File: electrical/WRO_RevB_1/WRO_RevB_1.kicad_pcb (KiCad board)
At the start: 2 copper layers, 117.5 x 50.6 mm, 23 parts, among them J1 VCC, J2 Conn_01x04_Pin, J4 Conn_01x11_Pin, J5 Conn_01x11_Pin, J6 3v3, J8 Conn_01x04_Pin, SW1 EXEC_PRGM, SW2 PWR, U3 BOB-12009

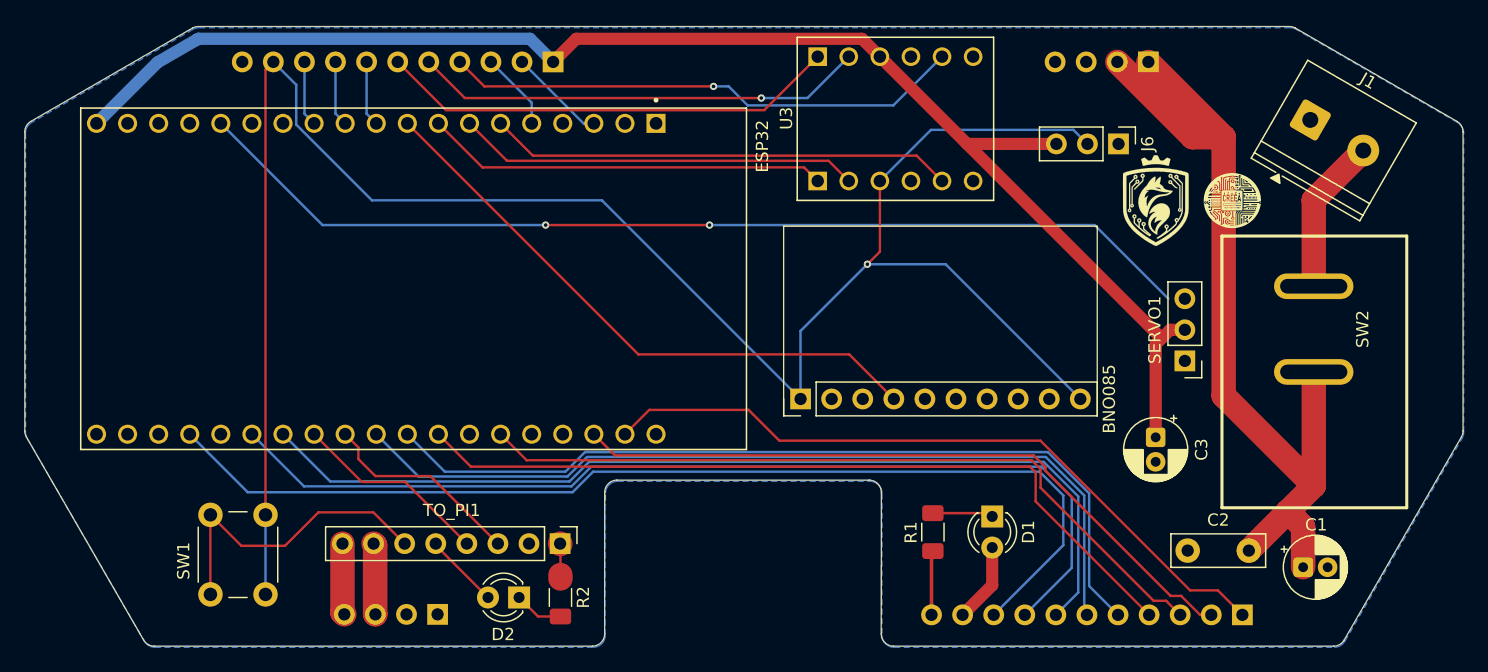
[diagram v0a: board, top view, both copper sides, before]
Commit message: actualiza PCB RevB
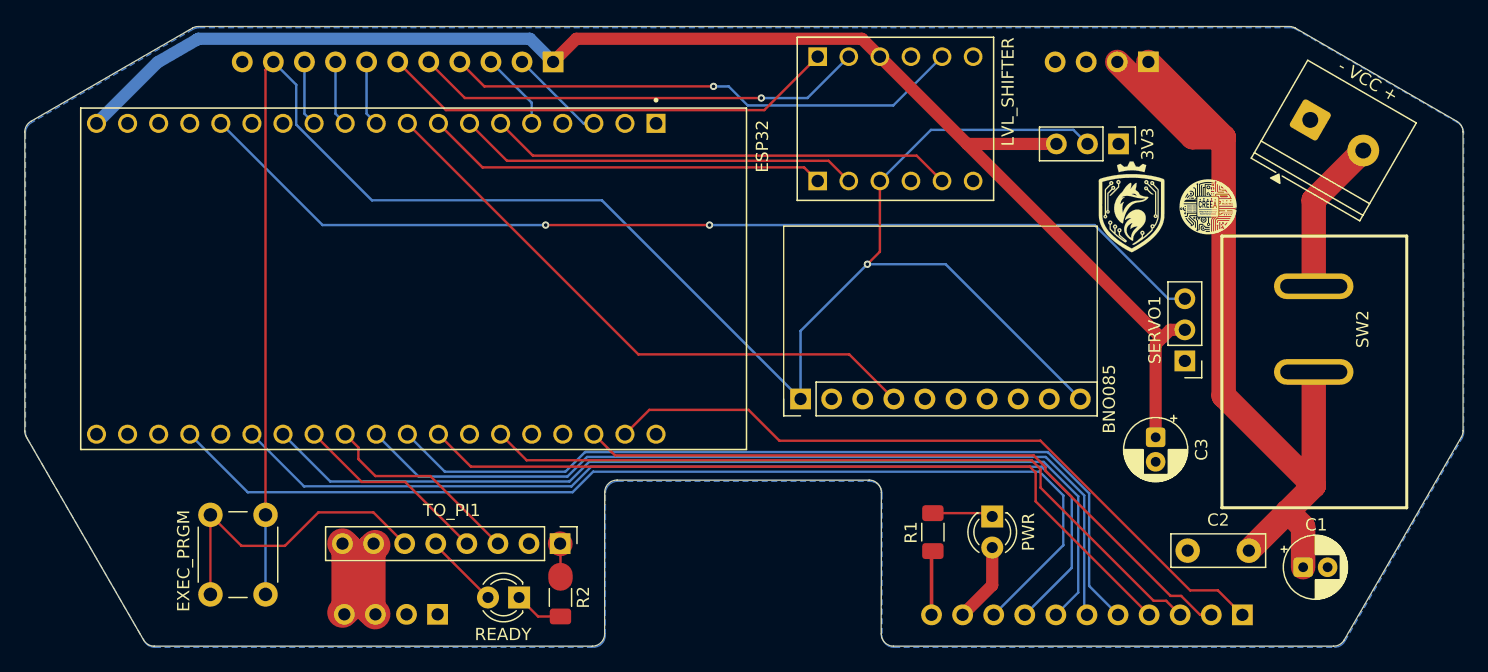
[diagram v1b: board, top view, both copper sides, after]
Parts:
- - VCC +: renamed from J1
- moved G*** 2.04 mm to (182.0, 81.5)
- moved G*** 2.04 mm to (188.2, 81.3)
- renumbered J6 to 3V3, SW1 to EXEC_PRGM, U3 to LVL_SHIFTER, D1 to PWR, D2 to READY
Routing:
- net SERVO: track 83.4 -> 84.7 mm
- net +5V_PI: track 11.7 -> 12.3 mm
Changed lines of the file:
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@@
 		(descr "Terminal Block Phoenix PT-1,5-2-5.0-H, 2 pins, pitch 5mm, size 10x9mm, drill diameter 1.3mm, pad diameter 2.6mm, http://www.mouser.com/ds/2/324/ItemDetail_1935161-922578.pdf")
 		(tags "THT Terminal Block Phoenix PT-1,5-2-5.0-H pitch 5mm size 10x9mm drill 1.3mm pad 2.6mm")
-		(property "Reference" "J1"
+		(property "Reference" "- VCC +"
 			(at 2.500001 -5.119999 150)
 			(layer "F.SilkS")
@@
 		(descr "Through hole straight pin header, 1x03, 2.54mm pitch, single row")
 		(tags "Through hole pin header THT 1x03 2.54mm single row")
-		(property "Reference" "J6"
+		(property "Reference" "3V3"
 			(at 0 -2.38 90)
 			(layer "F.SilkS")
@@
 		(layer "F.Cu")
 		(at 162.67 74.13 90)
-		(property "Reference" "U3"
-			(at 0.04 -8.9125 90)
+		(property "Reference" "LVL_SHIFTER"
+			(at 2.21 9.2 90)
 			(layer "F.SilkS")
 			(effects
@@
 	(footprint "LogoCREEA:LogoCREEA4.5"
 		(layer "F.Cu")
-		(at 190.22 80.812297)
+		(at 188.242289 81.319751)
 		(property "Reference" "G***"
 			(at 0 0 0)
@@
 		(descr "LED, diameter 3.0mm, 2 pins, generated by kicad-footprint-generator")
 		(tags "LED")
-		(property "Reference" "D2"
+		(property "Reference" "READY"
 			(at 1.31 -3.02 0)
 			(layer "F.SilkS")
@@
 		(descr "Generic 6mm SW tactile push button")
 		(tags "tact sw push 6mm")
-		(property "Reference" "SW1"
+		(property "Reference" "EXEC_PRGM"
 			(at 3.76 6.69 90)
 			(layer "F.SilkS")
@@
 	(footprint "LogoFoxR_2:LogoFoxR_2"
 		(layer "F.Cu")
-		(at 183.948975 80.959751)
+		(at 181.971264 81.467205)
 		(property "Reference" "G***"
 			(at 0 0 0)
@@
 		(descr "LED, diameter 3.0mm, 2 pins, generated by kicad-footprint-generator")
 		(tags "LED")
-		(property "Reference" "D1"
+		(property "Reference" "PWR"
 			(at 1.27 -2.96 90)
 			(layer "F.SilkS")
@@
 	)
 	(segment
-		(start 120.16 108.97)
-		(end 120.16 114.6)
-		(width 2)
+		(start 117.49 108.84)
+		(end 117.83 109.18)
+		(width 2.5)
+		(layer "F.Cu")
+		(net "+5V_PI")
+	)
+	(segment
+		(start 117.83 109.18)
+		(end 117.83 114.13)
+		(width 2.5)
+		(layer "F.Cu")
+		(net "+5V_PI")
+	)
+	(segment
+		(start 119.76 109.37)
+		(end 119.76 114.2)
+		(width 2.5)
 		(layer "F.Cu")
 		(net "+5V_PI")
@@
 	)
 	(segment
+		(start 117.83 114.13)
+		(end 117.49 114.47)
+		(width 2.5)
+		(layer "F.Cu")
+		(net "+5V_PI")
+	)
+	(segment
+		(start 120.16 108.97)
+		(end 119.76 109.37)
+		(width 2.5)
+		(layer "F.Cu")
+		(net "+5V_PI")
+	)
+	(segment
 		(start 117.49 114.47)
 		(end 117.64 114.62)
@@
 	)
 	(segment
-		(start 117.49 108.84)
-		(end 117.49 114.47)
-		(width 2)
+		(start 119.76 114.2)
+		(end 120.16 114.6)
+		(width 2.5)
 		(layer "F.Cu")
 		(net "+5V_PI")
 	)
 	(segment
+		(start 170.58 112.24)
+		(end 168.16 114.66)
+		(width 1)
+		(layer "F.Cu")
+		(net "+5V")
+	)
+	(segment
+		(start 184.35396 92.00396)
+		(end 168.53 76.18)
+		(width 1)
+		(layer "F.Cu")
+		(net "+5V")
+	)
+	(segment
+		(start 185.117919 91.37)
+		(end 186.32 91.37)
+		(width 1)
+		(layer "F.Cu")
+		(net "+5V")
+	)
+	(segment
+		(start 175.82 76.18)
+		(end 168.53 76.18)
+		(width 1)
+		(layer "F.Cu")
+		(net "+5V")
+	)
+	(segment
+		(start 184.48396 92.00396)
+		(end 184.35396 92.00396)
+		(width 1)
+		(layer "F.Cu")
+		(net "+5V")
+	)
+	(segment
+		(start 161.4 69.05)
+		(end 168.53 76.18)
+		(width 1)
+		(layer "F.Cu")
+		(net "+5V")
+	)
+	(segment
+		(start 170.58 109.16)
+		(end 170.58 112.24)
+		(width 1)
+		(layer "F.Cu")
+		(net "+5V")
+	)
+	(segment
+		(start 183.935 92.552919)
+		(end 184.48396 92.00396)
+		(width 1)
+		(layer "F.Cu")
+		(net "+5V")
+	)
+	(segment
+		(start 134.7 69.48)
+		(end 136.592 67.588)
+		(width 1)
+		(layer "F.Cu")
+		(net "+5V")
+	)
+	(segment
+		(start 183.935 100.154775)
+		(end 183.935 92.552919)
+		(width 1)
+		(layer "F.Cu")
+		(net "+5V")
+	)
+	(segment
+		(start 159.938 67.588)
+		(end 161.4 69.05)
+		(width 1)
+		(layer "F.Cu")
+		(net "+5V")
+	)
+	(segment
+		(start 136.592 67.588)
+		(end 159.938 67.588)
+		(width 1)
+		(layer "F.Cu")
+		(net "+5V")
+	)
+	(segment
+		(start 184.48396 92.00396)
+		(end 185.117919 91.37)
+		(width 1)
+		(layer "F.Cu")
+		(net "+5V")
+	)
+	(segment
+		(start 97.39 74.5)
+		(end 102.36696 69.52304)
+		(width 1)
+		(layer "B.Cu")
+		(net "+5V")
+	)
+	(segment
+		(start 105.706797 67.59974)
+		(end 105.719037 67.5875)
+		(width 1)
+		(layer "B.Cu")
+		(net "+5V")
+	)
+	(segment
+		(start 105.719037 67.5875)
+		(end 132.8075 67.5875)
+		(width 1)
+		(layer "B.Cu")
+		(net "+5V")
+	)
+	(segment
+		(start 102.36696 69.52304)
+		(end 105.559653 67.678985)
+		(width 1)
+		(layer "B.Cu")
+		(net "+5V")
+	)
+	(segment
+		(start 132.8075 67.5875)
+		(end 134.7 69.48)
+		(width 1)
+		(layer "B.Cu")
+		(net "+5V")
+	)
+	(segment
+		(start 105.559653 67.678985)
+		(end 105.706797 67.59974)
+		(width 1)
+		(layer "B.Cu")
+		(net "+5V")
+	)
+	(segment
 		(start 200.900127 76.72)
 		(end 196.85 80.770127)
@@
 	)
 	(segment
-		(start 178.95 82.81)
-		(end 147.48 82.81)
-		(width 0.2)
-		(layer "B.Cu")
-		(net "SERVO")
-	)
-	(segment
 		(start 134.09 82.81)
 		(end 115.86 82.81)
@@
 	)
 	(segment
-		(start 184.97 88.83)
-		(end 178.95 82.81)
+		(start 186.32 88.83)
+		(end 184.97 88.83)
 		(width 0.2)
 		(layer "B.Cu")
@@
 	)
 	(segment
-		(start 170.58 112.24)
-		(end 168.16 114.66)
-		(width 1)
-		(layer "F.Cu")
-		(net "+5V")
-	)
-	(segment
-		(start 184.35396 92.00396)
-		(end 168.53 76.18)
-		(width 1)
-		(layer "F.Cu")
-		(net "+5V")
-	)
-	(segment
-		(start 185.117919 91.37)
-		(end 186.32 91.37)
-		(width 1)
-		(layer "F.Cu")
-		(net "+5V")
-	)
-	(segment
-		(start 175.82 76.18)
-		(end 168.53 76.18)
-		(width 1)
-		(layer "F.Cu")
-		(net "+5V")
-	)
-	(segment
-		(start 184.48396 92.00396)
-		(end 184.35396 92.00396)
-		(width 1)
-		(layer "F.Cu")
-		(net "+5V")
-	)
-	(segment
-		(start 161.4 69.05)
-		(end 168.53 76.18)
-		(width 1)
-		(layer "F.Cu")
-		(net "+5V")
-	)
-	(segment
-		(start 170.58 109.16)
-		(end 170.58 112.24)
-		(width 1)
-		(layer "F.Cu")
-		(net "+5V")
-	)
-	(segment
-		(start 183.935 92.552919)
-		(end 184.48396 92.00396)
-		(width 1)
-		(layer "F.Cu")
-		(net "+5V")
-	)
-	(segment
-		(start 134.7 69.48)
-		(end 136.592 67.588)
-		(width 1)
-		(layer "F.Cu")
-		(net "+5V")
-	)
-	(segment
-		(start 183.935 100.154775)
-		(end 183.935 92.552919)
-		(width 1)
-		(layer "F.Cu")
-		(net "+5V")
-	)
-	(segment
-		(start 159.938 67.588)
-		(end 161.4 69.05)
-		(width 1)
-		(layer "F.Cu")
-		(net "+5V")
-	)
-	(segment
-		(start 136.592 67.588)
-		(end 159.938 67.588)
-		(width 1)
-		(layer "F.Cu")
-		(net "+5V")
-	)
-	(segment
-		(start 184.48396 92.00396)
-		(end 185.117919 91.37)
-		(width 1)
-		(layer "F.Cu")
-		(net "+5V")
-	)
-	(segment
-		(start 97.39 74.5)
-		(end 102.36696 69.52304)
-		(width 1)
-		(layer "B.Cu")
-		(net "+5V")
-	)
-	(segment
-		(start 105.706797 67.59974)
-		(end 105.719037 67.5875)
-		(width 1)
-		(layer "B.Cu")
-		(net "+5V")
-	)
-	(segment
-		(start 105.719037 67.5875)
-		(end 132.8075 67.5875)
-		(width 1)
-		(layer "B.Cu")
-		(net "+5V")
-	)
-	(segment
-		(start 102.36696 69.52304)
-		(end 105.559653 67.678985)
-		(width 1)
-		(layer "B.Cu")
-		(net "+5V")
-	)
-	(segment
-		(start 132.8075 67.5875)
-		(end 134.7 69.48)
-		(width 1)
+		(start 184.97 88.83)
+		(end 178.95 82.81)
+		(width 0.2)
 		(layer "B.Cu")
-		(net "+5V")
+		(net "SERVO")
 	)
 	(segment
-		(start 105.559653 67.678985)
-		(end 105.706797 67.59974)
-		(width 1)
+		(start 178.95 82.81)
+		(end 147.48 82.81)
+		(width 0.2)
 		(layer "B.Cu")
-		(net "+5V")
+		(net "SERVO")
 	)
 	(segment

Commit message: Revert "Merge branch 'main' of https://github.com/Nakashima26/WRO_FE_2026_FoxRobotics"
This reverts commit 232f9ecb01216201165b5abf43ae09e229c3eea8, reversing
changes made to 212c0f9856f89e84f48e320d89d4fd8fc24ab9e3.
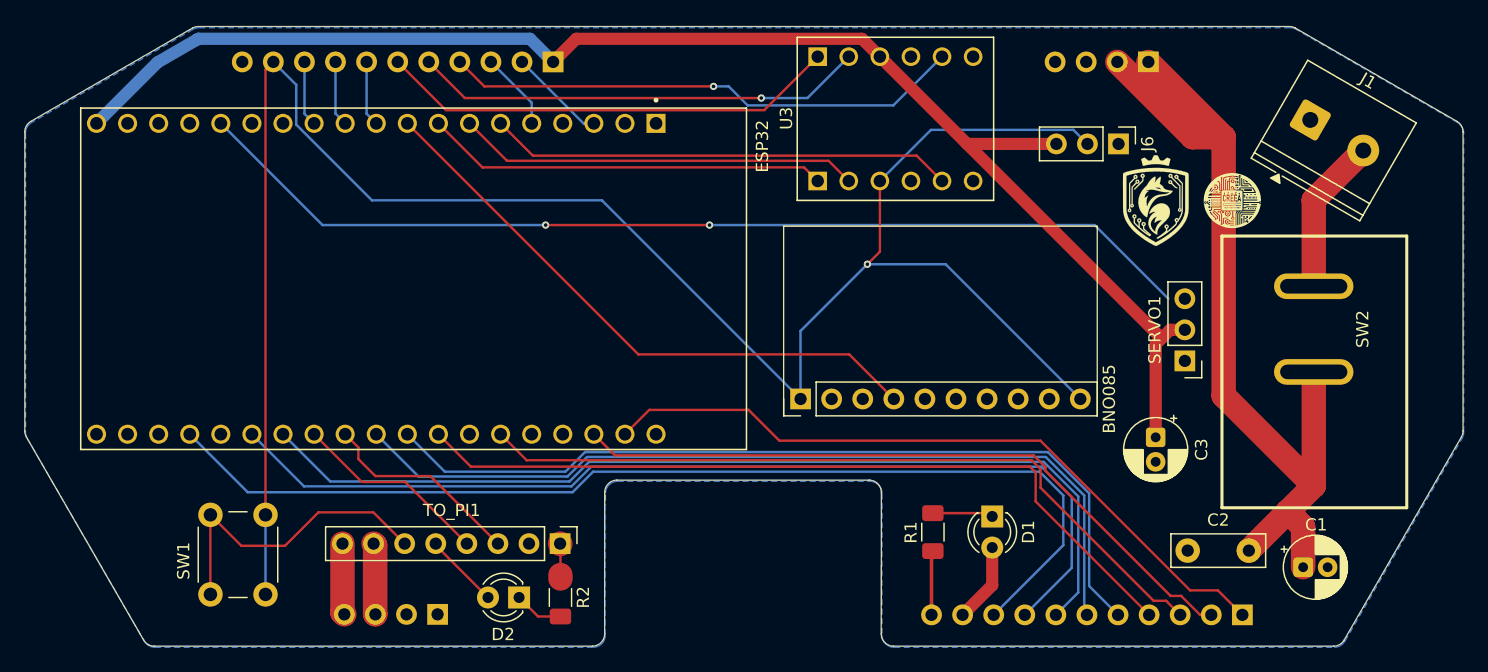
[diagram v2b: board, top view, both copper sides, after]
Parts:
- J1: renamed from - VCC +
- moved G*** 2.04 mm to (183.9, 81.0)
- moved G*** 2.04 mm to (190.2, 80.8)
- renumbered PWR to D1, READY to D2, 3V3 to J6, EXEC_PRGM to SW1, LVL_SHIFTER to U3
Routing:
- net SERVO: track 84.7 -> 83.4 mm
- net +5V_PI: track 12.3 -> 11.7 mm
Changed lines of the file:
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@@
 		(descr "Terminal Block Phoenix PT-1,5-2-5.0-H, 2 pins, pitch 5mm, size 10x9mm, drill diameter 1.3mm, pad diameter 2.6mm, http://www.mouser.com/ds/2/324/ItemDetail_1935161-922578.pdf")
 		(tags "THT Terminal Block Phoenix PT-1,5-2-5.0-H pitch 5mm size 10x9mm drill 1.3mm pad 2.6mm")
-		(property "Reference" "- VCC +"
+		(property "Reference" "J1"
 			(at 2.500001 -5.119999 150)
 			(layer "F.SilkS")
@@
 		(descr "Through hole straight pin header, 1x03, 2.54mm pitch, single row")
 		(tags "Through hole pin header THT 1x03 2.54mm single row")
-		(property "Reference" "3V3"
+		(property "Reference" "J6"
 			(at 0 -2.38 90)
 			(layer "F.SilkS")
@@
 		(layer "F.Cu")
 		(at 162.67 74.13 90)
-		(property "Reference" "LVL_SHIFTER"
-			(at 2.21 9.2 90)
+		(property "Reference" "U3"
+			(at 0.04 -8.9125 90)
 			(layer "F.SilkS")
 			(effects
@@
 	(footprint "LogoCREEA:LogoCREEA4.5"
 		(layer "F.Cu")
-		(at 188.242289 81.319751)
+		(at 190.22 80.812297)
 		(property "Reference" "G***"
 			(at 0 0 0)
@@
 		(descr "LED, diameter 3.0mm, 2 pins, generated by kicad-footprint-generator")
 		(tags "LED")
-		(property "Reference" "READY"
+		(property "Reference" "D2"
 			(at 1.31 -3.02 0)
 			(layer "F.SilkS")
@@
 		(descr "Generic 6mm SW tactile push button")
 		(tags "tact sw push 6mm")
-		(property "Reference" "EXEC_PRGM"
+		(property "Reference" "SW1"
 			(at 3.76 6.69 90)
 			(layer "F.SilkS")
@@
 	(footprint "LogoFoxR_2:LogoFoxR_2"
 		(layer "F.Cu")
-		(at 181.971264 81.467205)
+		(at 183.948975 80.959751)
 		(property "Reference" "G***"
 			(at 0 0 0)
@@
 		(descr "LED, diameter 3.0mm, 2 pins, generated by kicad-footprint-generator")
 		(tags "LED")
-		(property "Reference" "PWR"
+		(property "Reference" "D1"
 			(at 1.27 -2.96 90)
 			(layer "F.SilkS")
@@
 	)
 	(segment
-		(start 117.49 108.84)
-		(end 117.83 109.18)
-		(width 2.5)
-		(layer "F.Cu")
-		(net "+5V_PI")
-	)
-	(segment
-		(start 117.83 109.18)
-		(end 117.83 114.13)
-		(width 2.5)
-		(layer "F.Cu")
-		(net "+5V_PI")
-	)
-	(segment
-		(start 119.76 109.37)
-		(end 119.76 114.2)
-		(width 2.5)
+		(start 120.16 108.97)
+		(end 120.16 114.6)
+		(width 2)
 		(layer "F.Cu")
 		(net "+5V_PI")
@@
 	)
 	(segment
-		(start 117.83 114.13)
-		(end 117.49 114.47)
-		(width 2.5)
-		(layer "F.Cu")
-		(net "+5V_PI")
-	)
-	(segment
-		(start 120.16 108.97)
-		(end 119.76 109.37)
-		(width 2.5)
-		(layer "F.Cu")
-		(net "+5V_PI")
-	)
-	(segment
 		(start 117.49 114.47)
 		(end 117.64 114.62)
@@
 	)
 	(segment
-		(start 119.76 114.2)
-		(end 120.16 114.6)
-		(width 2.5)
+		(start 117.49 108.84)
+		(end 117.49 114.47)
+		(width 2)
 		(layer "F.Cu")
 		(net "+5V_PI")
 	)
 	(segment
-		(start 170.58 112.24)
-		(end 168.16 114.66)
-		(width 1)
-		(layer "F.Cu")
-		(net "+5V")
-	)
-	(segment
-		(start 184.35396 92.00396)
-		(end 168.53 76.18)
-		(width 1)
-		(layer "F.Cu")
-		(net "+5V")
-	)
-	(segment
-		(start 185.117919 91.37)
-		(end 186.32 91.37)
-		(width 1)
-		(layer "F.Cu")
-		(net "+5V")
-	)
-	(segment
-		(start 175.82 76.18)
-		(end 168.53 76.18)
-		(width 1)
-		(layer "F.Cu")
-		(net "+5V")
-	)
-	(segment
-		(start 184.48396 92.00396)
-		(end 184.35396 92.00396)
-		(width 1)
-		(layer "F.Cu")
-		(net "+5V")
-	)
-	(segment
-		(start 161.4 69.05)
-		(end 168.53 76.18)
-		(width 1)
-		(layer "F.Cu")
-		(net "+5V")
-	)
-	(segment
-		(start 170.58 109.16)
-		(end 170.58 112.24)
-		(width 1)
-		(layer "F.Cu")
-		(net "+5V")
-	)
-	(segment
-		(start 183.935 92.552919)
-		(end 184.48396 92.00396)
-		(width 1)
-		(layer "F.Cu")
-		(net "+5V")
-	)
-	(segment
-		(start 134.7 69.48)
-		(end 136.592 67.588)
-		(width 1)
-		(layer "F.Cu")
-		(net "+5V")
-	)
-	(segment
-		(start 183.935 100.154775)
-		(end 183.935 92.552919)
-		(width 1)
-		(layer "F.Cu")
-		(net "+5V")
-	)
-	(segment
-		(start 159.938 67.588)
-		(end 161.4 69.05)
-		(width 1)
-		(layer "F.Cu")
-		(net "+5V")
-	)
-	(segment
-		(start 136.592 67.588)
-		(end 159.938 67.588)
-		(width 1)
-		(layer "F.Cu")
-		(net "+5V")
-	)
-	(segment
-		(start 184.48396 92.00396)
-		(end 185.117919 91.37)
-		(width 1)
-		(layer "F.Cu")
-		(net "+5V")
-	)
-	(segment
-		(start 97.39 74.5)
-		(end 102.36696 69.52304)
-		(width 1)
-		(layer "B.Cu")
-		(net "+5V")
-	)
-	(segment
-		(start 105.706797 67.59974)
-		(end 105.719037 67.5875)
-		(width 1)
-		(layer "B.Cu")
-		(net "+5V")
-	)
-	(segment
-		(start 105.719037 67.5875)
-		(end 132.8075 67.5875)
-		(width 1)
-		(layer "B.Cu")
-		(net "+5V")
-	)
-	(segment
-		(start 102.36696 69.52304)
-		(end 105.559653 67.678985)
-		(width 1)
-		(layer "B.Cu")
-		(net "+5V")
-	)
-	(segment
-		(start 132.8075 67.5875)
-		(end 134.7 69.48)
-		(width 1)
-		(layer "B.Cu")
-		(net "+5V")
-	)
-	(segment
-		(start 105.559653 67.678985)
-		(end 105.706797 67.59974)
-		(width 1)
-		(layer "B.Cu")
-		(net "+5V")
-	)
-	(segment
 		(start 200.900127 76.72)
 		(end 196.85 80.770127)
@@
 	)
 	(segment
-		(start 134.09 82.81)
-		(end 115.86 82.81)
+		(start 178.95 82.81)
+		(end 147.48 82.81)
 		(width 0.2)
 		(layer "B.Cu")
@@
 	)
 	(segment
-		(start 115.86 82.81)
-		(end 107.55 74.5)
+		(start 134.09 82.81)
+		(end 115.86 82.81)
 		(width 0.2)
 		(layer "B.Cu")
@@
 	)
 	(segment
-		(start 186.32 88.83)
-		(end 184.97 88.83)
+		(start 115.86 82.81)
+		(end 107.55 74.5)
 		(width 0.2)
 		(layer "B.Cu")
@@
 	)
 	(segment
-		(start 178.95 82.81)
-		(end 147.48 82.81)
-		(width 0.2)
+		(start 170.58 112.24)
+		(end 168.16 114.66)
+		(width 1)
+		(layer "F.Cu")
+		(net "+5V")
+	)
+	(segment
+		(start 184.35396 92.00396)
+		(end 168.53 76.18)
+		(width 1)
+		(layer "F.Cu")
+		(net "+5V")
+	)
+	(segment
+		(start 185.117919 91.37)
+		(end 186.32 91.37)
+		(width 1)
+		(layer "F.Cu")
+		(net "+5V")
+	)
+	(segment
+		(start 175.82 76.18)
+		(end 168.53 76.18)
+		(width 1)
+		(layer "F.Cu")
+		(net "+5V")
+	)
+	(segment
+		(start 184.48396 92.00396)
+		(end 184.35396 92.00396)
+		(width 1)
+		(layer "F.Cu")
+		(net "+5V")
+	)
+	(segment
+		(start 161.4 69.05)
+		(end 168.53 76.18)
+		(width 1)
+		(layer "F.Cu")
+		(net "+5V")
+	)
+	(segment
+		(start 170.58 109.16)
+		(end 170.58 112.24)
+		(width 1)
+		(layer "F.Cu")
+		(net "+5V")
+	)
+	(segment
+		(start 183.935 92.552919)
+		(end 184.48396 92.00396)
+		(width 1)
+		(layer "F.Cu")
+		(net "+5V")
+	)
+	(segment
+		(start 134.7 69.48)
+		(end 136.592 67.588)
+		(width 1)
+		(layer "F.Cu")
+		(net "+5V")
+	)
+	(segment
+		(start 183.935 100.154775)
+		(end 183.935 92.552919)
+		(width 1)
+		(layer "F.Cu")
+		(net "+5V")
+	)
+	(segment
+		(start 159.938 67.588)
+		(end 161.4 69.05)
+		(width 1)
+		(layer "F.Cu")
+		(net "+5V")
+	)
+	(segment
+		(start 136.592 67.588)
+		(end 159.938 67.588)
+		(width 1)
+		(layer "F.Cu")
+		(net "+5V")
+	)
+	(segment
+		(start 184.48396 92.00396)
+		(end 185.117919 91.37)
+		(width 1)
+		(layer "F.Cu")
+		(net "+5V")
+	)
+	(segment
+		(start 97.39 74.5)
+		(end 102.36696 69.52304)
+		(width 1)
 		(layer "B.Cu")
-		(net "SERVO")
+		(net "+5V")
+	)
+	(segment
+		(start 105.706797 67.59974)
+		(end 105.719037 67.5875)
+		(width 1)
+		(layer "B.Cu")
+		(net "+5V")
+	)
+	(segment
+		(start 105.719037 67.5875)
+		(end 132.8075 67.5875)
+		(width 1)
+		(layer "B.Cu")
+		(net "+5V")
+	)
+	(segment
+		(start 102.36696 69.52304)
+		(end 105.559653 67.678985)
+		(width 1)
+		(layer "B.Cu")
+		(net "+5V")
+	)
+	(segment
+		(start 132.8075 67.5875)
+		(end 134.7 69.48)
+		(width 1)
+		(layer "B.Cu")
+		(net "+5V")
+	)
+	(segment
+		(start 105.559653 67.678985)
+		(end 105.706797 67.59974)
+		(width 1)
+		(layer "B.Cu")
+		(net "+5V")
 	)
 	(segment
